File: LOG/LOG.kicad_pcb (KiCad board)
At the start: 2 copper layers, 30.5 x 17.8 mm, 16 parts, among them J1 Micro_SD_Card_Det, U1 DS3231MZ

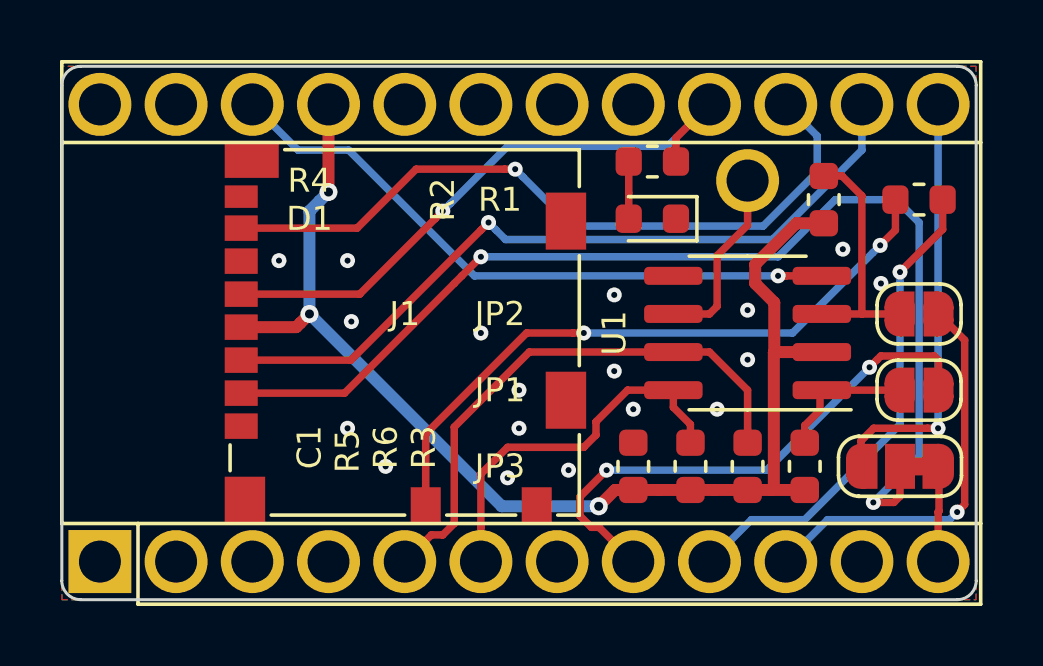
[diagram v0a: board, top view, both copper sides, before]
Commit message: major cleanup and fixes
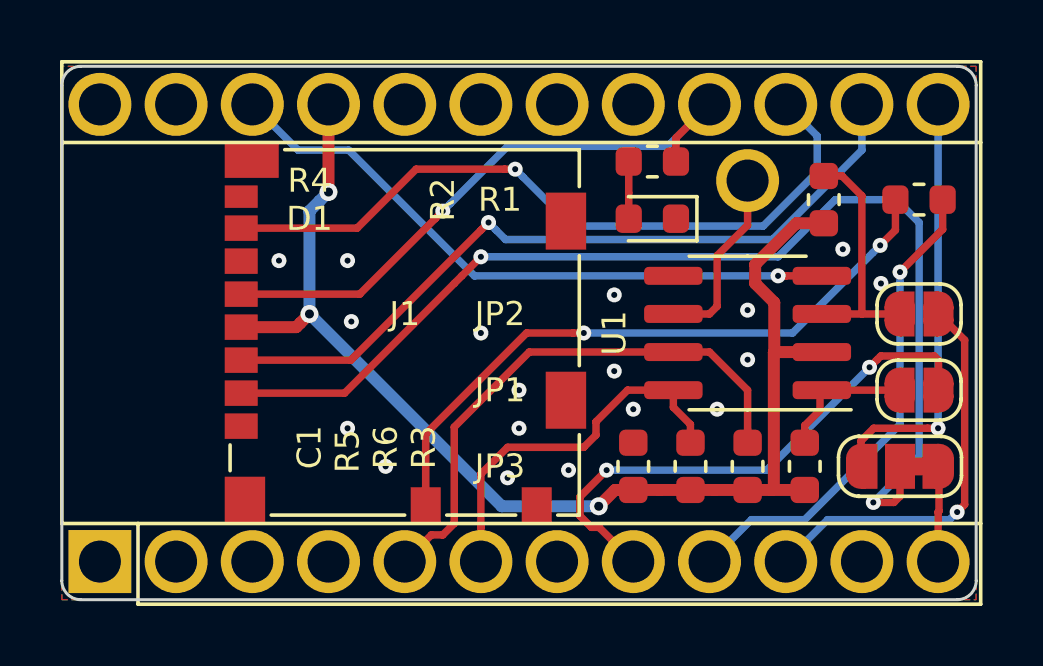
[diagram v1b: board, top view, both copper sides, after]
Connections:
- net ~RST renamed ~{RST}
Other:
- net class Default removed
- net class Power removed
- net class small removed
- net class tiny removed
